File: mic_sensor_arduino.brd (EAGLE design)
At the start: 13.3 x 29.6 mm, 19 parts, among them U1 LM393DR, U2 LM393DR

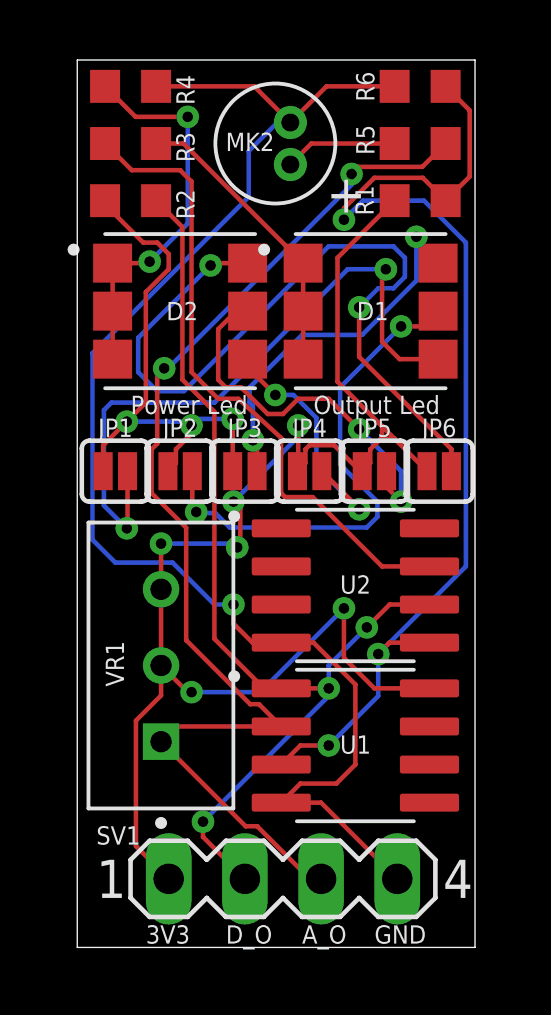
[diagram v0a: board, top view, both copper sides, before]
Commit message: update resources
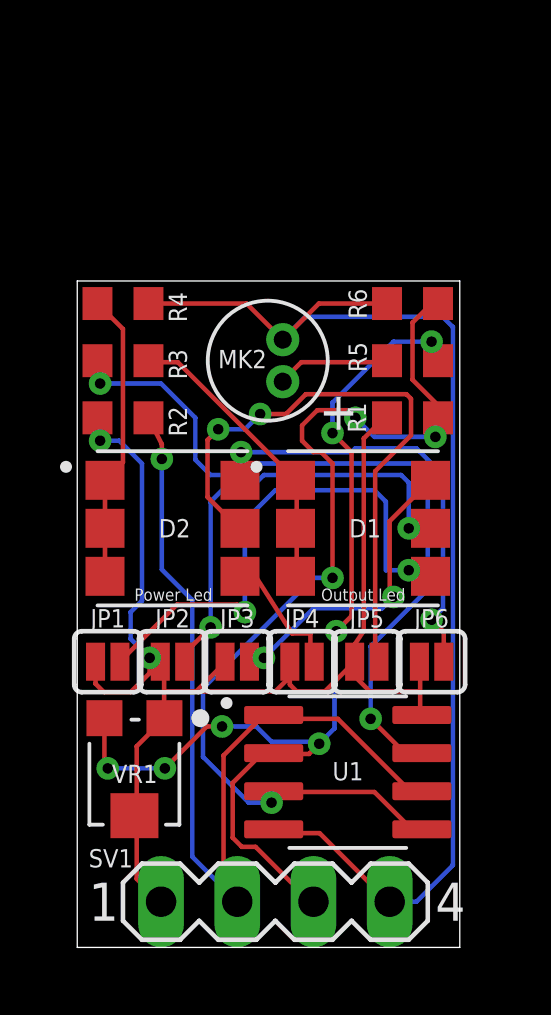
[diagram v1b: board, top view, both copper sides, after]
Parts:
- removed U2: LM393DR, LM393DR:SOIC127P599X175-8N
- VR1: value 3296W-1-103RLF -> TC33X-2-103G; device 3296W-1-103RLF:TRIM_3296W-1-103RLF -> TC33X-2-103G:TRIMMER_TC33X-2-103G
- moved MK2 7.24 mm to (6.35, 19.6)
- moved R1 7.24 mm to (11.2, 17.7)
- moved R2 7.24 mm to (1.52, 17.7)
- moved R3 7.24 mm to (1.52, 19.6)
- moved R4 7.24 mm to (1.52, 21.5)
- moved R5 7.24 mm to (11.2, 19.6)
- moved R6 7.24 mm to (11.2, 21.5)
- moved D1 7.24 mm to (9.53, 14.0)
- moved D2 7.24 mm to (3.17, 14.0)
- moved JP1 6.36 mm to (1.02, 9.53)
- moved JP2 6.36 mm to (3.17, 9.53)
- moved JP3 6.36 mm to (5.33, 9.53)
- moved JP4 6.36 mm to (7.49, 9.53)
- moved JP5 6.36 mm to (9.65, 9.53)
- moved JP6 6.36 mm to (11.8, 9.53)
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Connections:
- removed net VCC: U2.8
- net 2IN+: now also U1.5; no longer U2.5
- net 2OUT: now also U1.7; no longer U2.7
- net 3V3: now also VR1.1; no longer VR1.3
- net A_OUT: now also VR1.3; no longer VR1.1
- net D_OUT: now also U1.6; no longer U2.6
- net GND: no longer U2.4
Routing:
- net 3V3: track 69.6 -> 45.1 mm, vias 9 -> 2
- net N$8: track 26.4 -> 14.7 mm
- net N$7: track 12.9 -> 20.2 mm
- net GND: track 47.6 -> 40.6 mm, vias 1 -> 0
- net N$1: track 22.1 -> 17.7 mm
- net N$6: track 8.68 -> 4.44 mm, vias 2 -> 0
- net 2OUT: track 21.4 -> 25.1 mm, vias 0 -> 2
- net 2IN+: track 36.3 -> 32.9 mm, vias 3 -> 4
- net P_L_GND: track 13.0 -> 9.69 mm, vias 2 -> 0
- net D_OUT: track 33.5 -> 30.7 mm, vias 3 -> 1
- net A_OUT: track 38.2 -> 35.5 mm, vias 2 -> 7
- net N$5: track 12.6 -> 10.2 mm
- net N$2: track 17.0 -> 15.1 mm
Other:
- board size 13.3 x 29.6 mm -> 12.8 x 22.2 mm
- board text added: "LM393 Sound Sensor v1.0 by DoganM95"
- board text removed: "v0.9 by DoganM95"
